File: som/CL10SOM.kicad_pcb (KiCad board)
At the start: 4 copper layers, 31 x 30.5 mm, 64 parts, among them IC1 10CL025YU256C8G, U1 MT46H32M16LFBF-5 IT:C, U2 MX25L12833FM2, U3 SC189ZSKTRT, U4 SC189CSKTRT, U6 AT93C46DN-SH-T, U7 SG3225CAN 50.0000M-TJGA6, U8 SG3225CAN 50.0000M-TJGA6, X1 DF40C-120DS-0.4V51

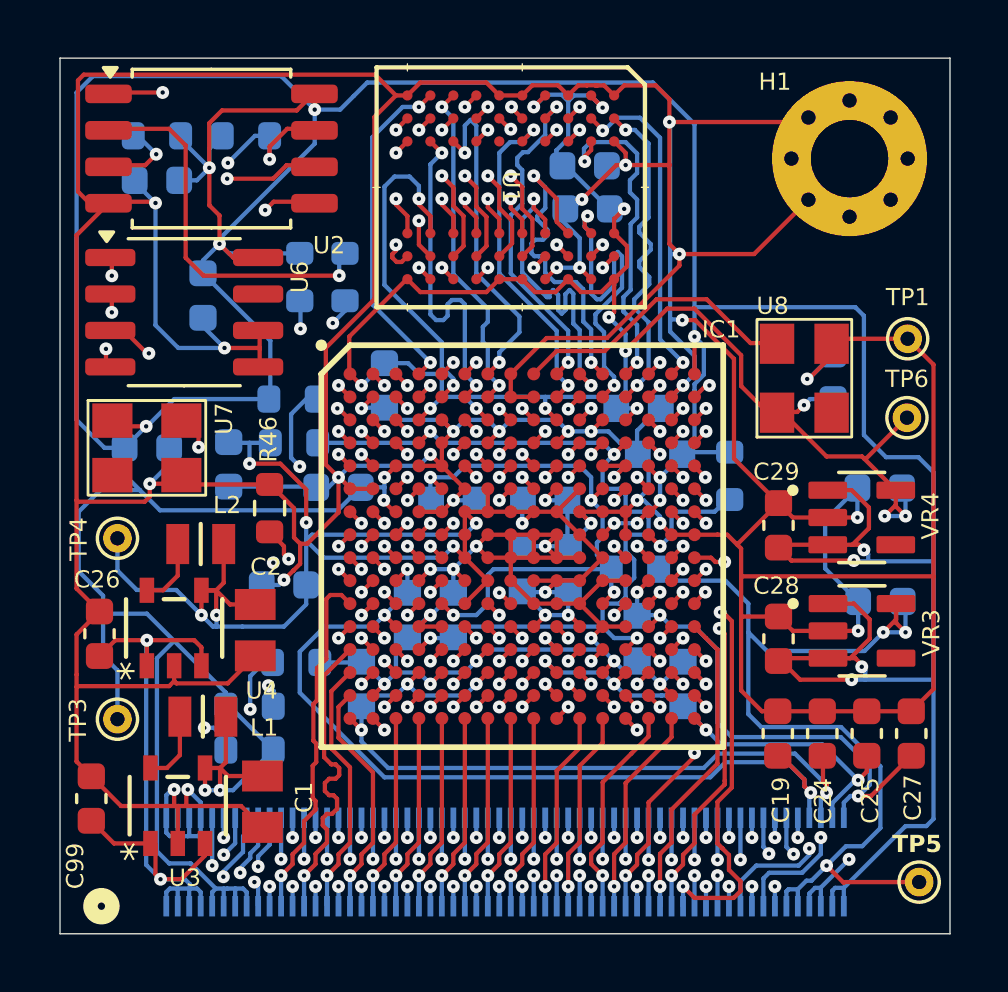
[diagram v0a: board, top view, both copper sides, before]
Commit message: Improvements
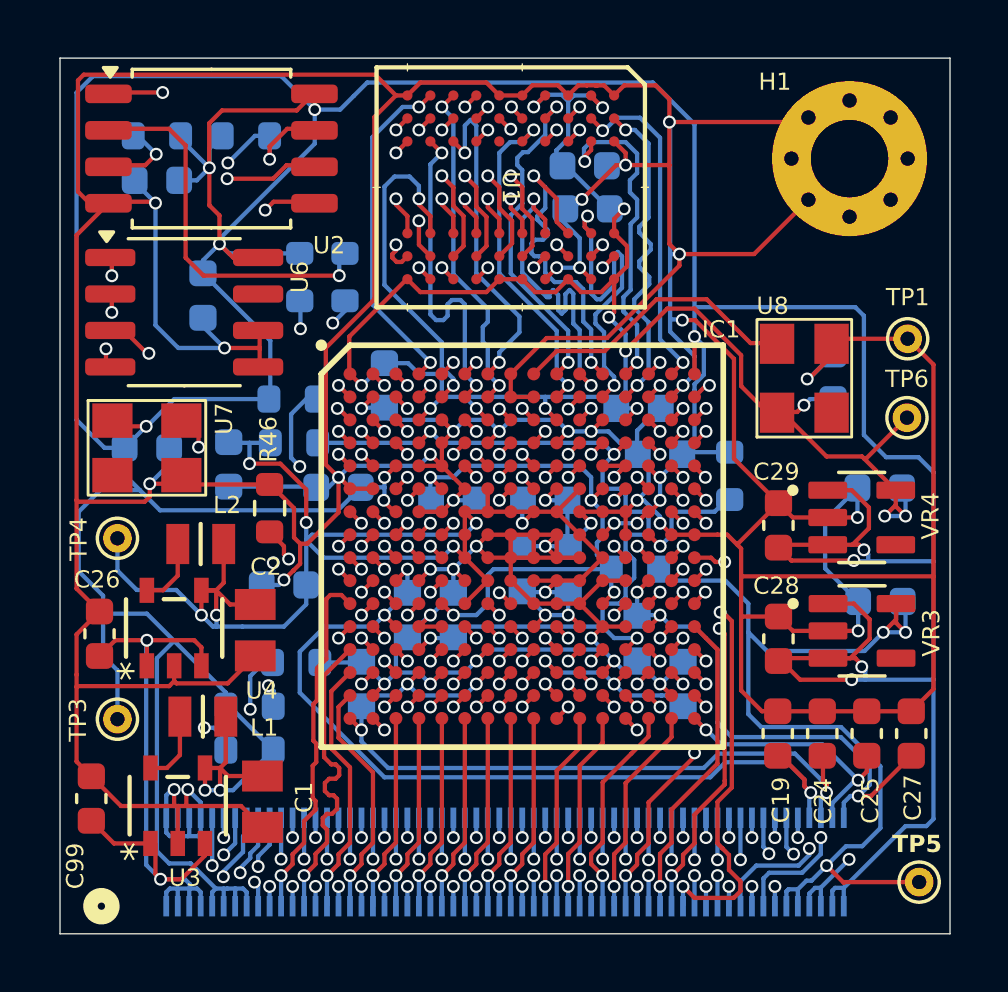
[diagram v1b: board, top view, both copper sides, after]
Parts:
- L1, L2: value MURATA_DFE21CCN1R0MELL -> DFE21CCN1R0MELL
- R62: value 25E -> 24E9
